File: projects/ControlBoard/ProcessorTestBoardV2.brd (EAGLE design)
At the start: 50.8 x 50.8 mm, 87 parts

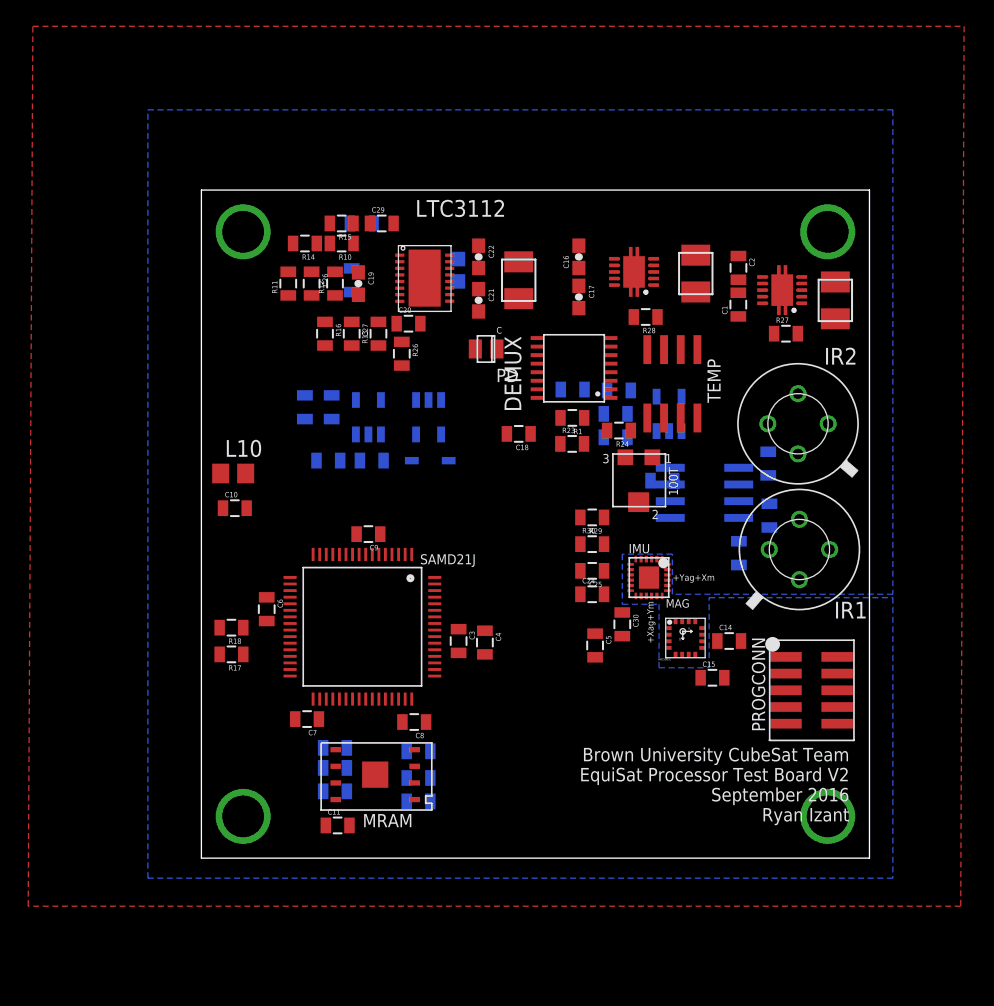
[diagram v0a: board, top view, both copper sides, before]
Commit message: Top and Side Panels, Proc Test Board prepared for production
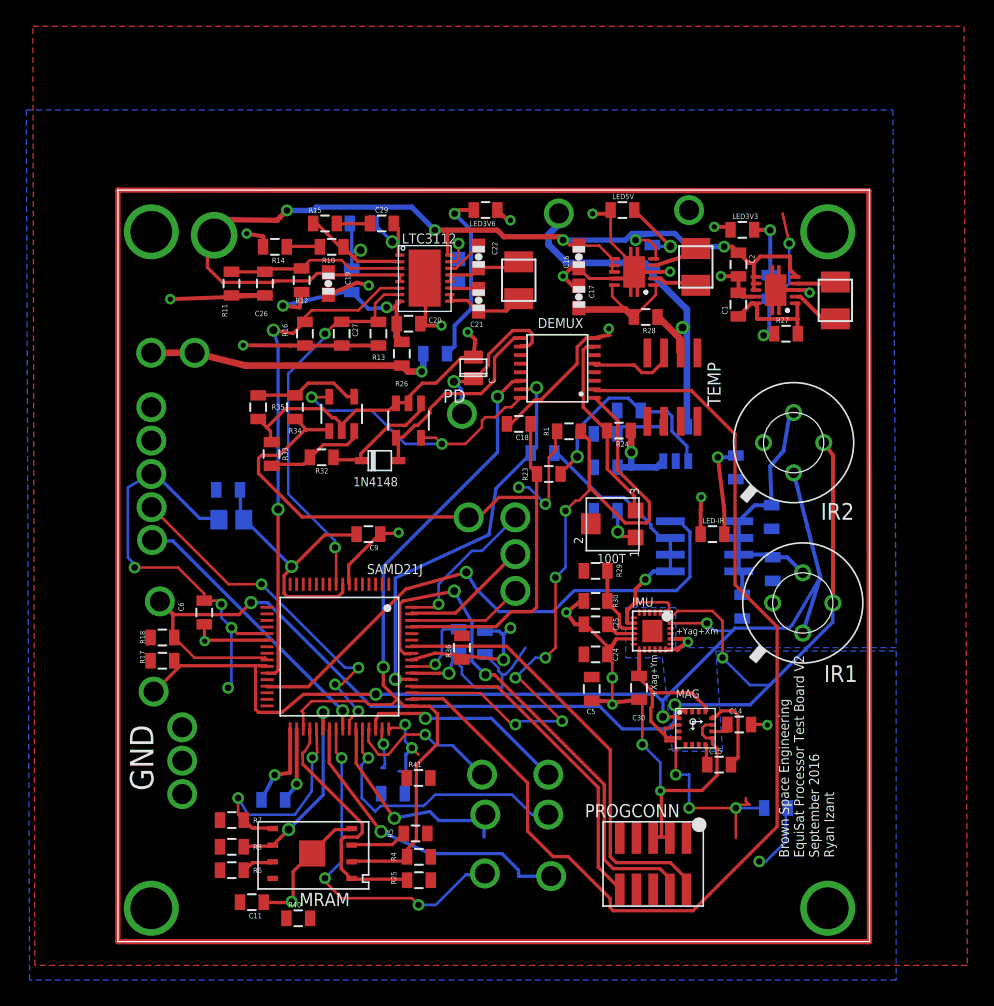
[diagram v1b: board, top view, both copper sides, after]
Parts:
- added LED-IR, LED3V3, LED3V6, LED5V: (no value), CNTRL_BOARD:0805
- added R31: 560R, CNTRL_BOARD:0805
- added R36, R40, R41, R42: 0R, CNTRL_BOARD:0805
- added R37, R38: 250R, CNTRL_BOARD:0805
- added R39: 330R, CNTRL_BOARD:0805
- moved PROGCONN 15.8 mm to (30.5, 1.52), turned to 0 degrees
- moved R6 9.87 mm to (2.31, -0.92), flipped to the top
- moved R8 9.87 mm to (2.31, 0.86), flipped to the top
- moved R7 9.57 mm to (2.31, 2.89), flipped to the top
- moved C11 8.75 mm to (3.84, -3.35), turned to 180 degrees
- moved MRAM 7.68 mm to (8.42, 0.35)
- moved MAG 6.90 mm to (36.1, 8.38)
- moved C7 6.66 mm to (5.46, 4.43), flipped to the bottom, turned to 0 degrees
- moved C15 6.62 mm to (39.4, 7.11)
- moved C14 6.40 mm to (40.9, 10.2)
- moved R5 6.25 mm to (16.3, 1.88), flipped to the top
- moved 100T 6.23 mm to (33.0, 24.4), turned to 90 degrees
- moved R4 6.00 mm to (16.5, 0.10), flipped to the top
- moved R25 6.00 mm to (16.5, -1.68), flipped to the top
- moved C8 5.69 mm to (14.6, 4.90), flipped to the bottom, turned to 0 degrees
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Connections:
- removed net PA10: SAMD21J.P$19
- new net N$16: LED-IR.2, R38.1
- new net N$21: LED3V6.2, R39.1
- new net N$22: LED5V.2, R31.1
- new net N$23: LED3V3.2, R37.1
- new net PA20[2]: SAMD21J.P$41
- new net PA21[3]: SAMD21J.P$42
- new net PA22: SAMD21J.P$43
- new net PA23: SAMD21J.P$44
- new net PA24: SAMD21J.P$45
- new net PA25: SAMD21J.P$46
- new net PAD[0]: SAMD21J.P$13
- new net PAD[1]: SAMD21J.P$14
- new net PB02: SAMD21J.P$63
- new net PB03: SAMD21J.P$64
- new net PB16: SAMD21J.P$39
- new net PB17: SAMD21J.P$40
- net 3V3: now also R36.1, R36.2, R37.2, R40.1, R40.2, R41.1, R41.2, R42.1, R42.2
- net 3V6: now also R39.2
- net 5V: now also R31.2
- net GND: now also LED-IR.1, LED3V3.1, LED3V6.1, LED5V.1
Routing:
- net N$20: track 0.00 -> 228.5 mm
- net GND: track 0.00 -> 198.6 mm, vias 4 -> 37
- net 3V3: track 0.00 -> 167.9 mm, vias 0 -> 22
- net SDA: track 0.00 -> 97.6 mm, vias 0 -> 4
- net VIN: track 0.00 -> 83.9 mm, vias 0 -> 6
- net S1: track 0.00 -> 83.0 mm
- net SCL: track 0.00 -> 82.1 mm, vias 0 -> 4
- net SO: track 0.00 -> 58.3 mm, vias 0 -> 2
- net ~1OE: track 0.00 -> 56.2 mm, vias 0 -> 6
- net PB00: track 0.00 -> 56.2 mm, vias 0 -> 1
- net PA12: track 0.00 -> 43.2 mm, vias 0 -> 1
- net PA30: track 0.00 -> 40.5 mm, vias 0 -> 2
- net RUN: track 0.00 -> 38.1 mm, vias 0 -> 2
- net PA31: track 0.00 -> 33.8 mm
- net ~2OE: track 0.00 -> 30.6 mm, vias 0 -> 2
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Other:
- board size 50.8 x 50.8 mm -> 57.1 x 57.1 mm
- board text added: "3V3"
- board text added: "3V6"
- board text added: "5V"
- board text added: "Brown Space Engineering EquiSat Processor Test Board V2 September 2016 Ryan Izant"
- board text added: "GND"
- board text added: "PA20[2]"
- board text added: "PA21[3]"
- board text added: "PA22"
- board text added: "PA23"
- board text added: "PA24"
- board text added: "PA25"
- board text added: "PB00"
- board text added: "PB01"
- board text added: "PB02"
- board text added: "PB03"
- board text added: "PB16"
- board text added: "PB17"
- board text added: "SCL"
- board text added: "SDA"
- board text added: "VIN"
- board text removed: "Brown University CubeSat Team EquiSat Processor Test Board V2 September 2016 Ryan Izant"

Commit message: Started Battery Board and fixes to library
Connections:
- net N$1: now also R38.2
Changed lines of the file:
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@@
 <wire x1="41.1226" y1="20.0262" x2="41.1226" y2="21.5424" width="0.3048" layer="16"/>
 <wire x1="41.1226" y1="21.5424" x2="40.856" y2="21.809" width="0.3048" layer="16"/>
+<contactref element="R38" pad="2"/>
+<wire x1="42.075" y1="26.838" x2="40.64" y2="28.818" width="0" layer="19" extent="16-16"/>
 </signal>
 <signal name="SDA">
